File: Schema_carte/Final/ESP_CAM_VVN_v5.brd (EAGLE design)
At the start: 55.2 x 60.8 mm, 66 parts, among them M1 ELECTRET_MICROPHON-WM-62PC/62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, Q1 SI2305CDS, Q2 BSS131, Q3 SI2305CDS, Q6 SI2305CDS, Q7 BSS131, Q8 BSS131, U1 MCP3428-E/SL, U2 ESP32-WROVER-E, U3 PCA9685PW, U4 MIC5239-ADJMM, U5 MIC5239S, U6 MIC5239-ADJMM, X1 B2B-PH-K-S, X2 FH12-24S-0.5SH

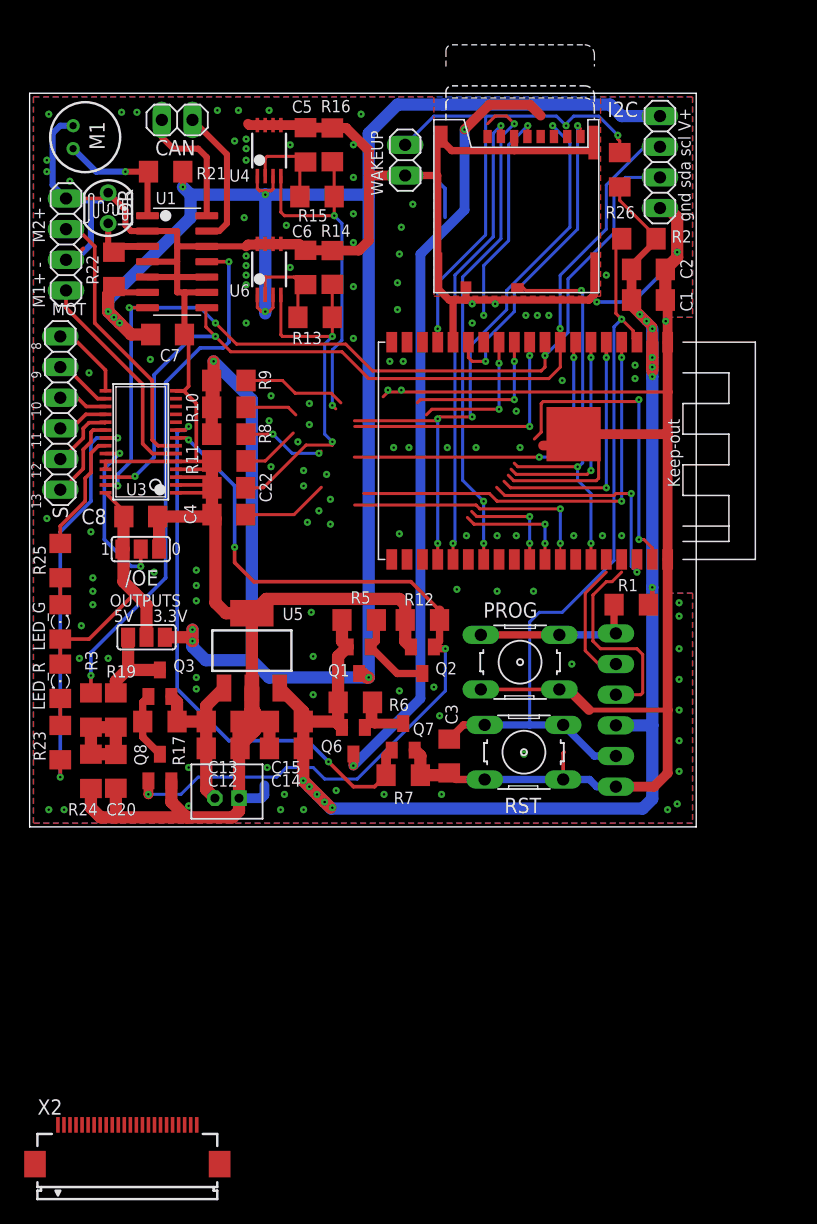
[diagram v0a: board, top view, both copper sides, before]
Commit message: romain maj
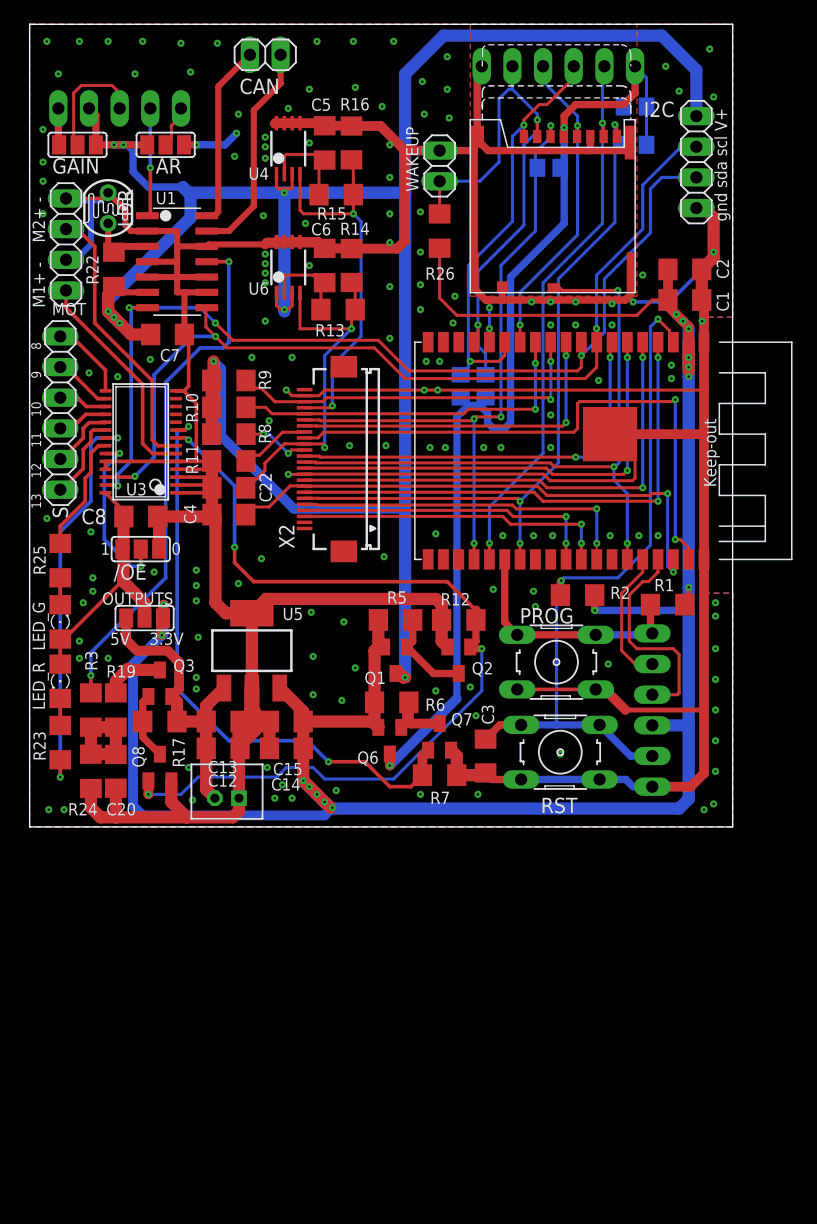
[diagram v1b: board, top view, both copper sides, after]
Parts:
- removed M1: ELECTRET_MICROPHON-WM-62PC/62PK, microphon:WM-62PC/62PK
- added AR, GAIN: (no value), jumper:SJ_2
- added MAX9814: (no value), pinhead:1X05
- added R18, R20, R27, R4: 47k, rcl:R0805
- added SD_SPI: (no value), pinhead:1X06
- R21: value 10k -> 47k; device eagle-ltspice:R1206 -> rcl:R0805
- moved X2 61.1 mm to (26.0, 30.5), turned to 90 degrees
- moved R21 39.3 mm to (50.2, 59.7), flipped to the bottom
- moved R2 30.0 mm to (45.4, 19.2)
- moved R26 15.8 mm to (34.0, 49.4)
- moved CAN 9.08 mm to (19.5, 64.0)
- moved R1 3.02 mm to (52.9, 18.4)
- moved C1 3.02 mm to (54.3, 43.7)
- moved C2 3.02 mm to (54.3, 46.2)
- moved C3 3.02 mm to (37.8, 5.87)
- moved I2C 3.02 mm to (55.2, 55.1)
- moved JP6 3.02 mm to (55.4, 9.68)
- moved PROG 3.02 mm to (43.7, 13.7)
- moved Q1 3.02 mm to (30.3, 13.8)
- moved Q2 3.02 mm to (35.6, 13.8)
- moved Q6 3.02 mm to (29.8, 7.14)
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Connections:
- removed net N$11: M1.2, R21.1, U1.1
- removed net SD_CLK: SD1.P$4
- new net AR: AR.2, MAX9814.1
- new net GAIN: GAIN.2, MAX9814.3
- new net N$2: MAX9814.2, U1.1
- net +5V: now also OUTPUTS.1
- net +5V/1: no longer OUTPUTS.1
- net CA_D0_SD_D1: now also R20.2
- net CA_PWDN_SD_CLK: now also SD1.P$4, SD_SPI.4
- net CA_RST_SD_CMD: now also R27.2
- net GND: now also AR.3, GAIN.1, MAX9814.5, SD_SPI.6; no longer M1.1
- net IO0: now also U2.IO0
- net RX: now also U2.RXD0; no longer U2.TXD0
- net SD_D0: now also R21.2, SD_SPI.2
- net SD_D2: now also R18.2, SD_SPI.3
- net SD_D3: now also R4.2, SD_SPI.5
- net TX: now also U2.TXD0; no longer U2.RXD0
- net V+: now also AR.1, GAIN.3, MAX9814.4; no longer OUTPUTS.3, R21.2
- net V+_SD: now also R18.1, R20.1, R21.1, R27.1, R4.1, SD_SPI.1
- net VCC: now also OUTPUTS.3
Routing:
- net VCC: track 118.2 -> 186.3 mm, vias 12 -> 15
- net GND: track 423.0 -> 452.0 mm, vias 124 -> 152
- net CA_PWDN_SD_CLK: track 0.00 -> 26.9 mm, vias 0 -> 2
- net CA_HREF: track 25.3 -> 47.2 mm
- net CA_XCLK_SD_DET: track 33.8 -> 54.2 mm
- net CA_D6: track 17.6 -> 37.7 mm
- net CA_D5: track 20.8 -> 40.3 mm
- net CA_D0_SD_D1: track 41.6 -> 59.4 mm
- net CA_PCLK: track 26.5 -> 44.1 mm
- net CA_D1: track 8.54 -> 25.4 mm
- net CA_D2: track 9.58 -> 26.1 mm
- net CA_SIO_C: track 16.2 -> 29.9 mm
- net N$11: track 10.7 -> 0.00 mm, vias 1 -> 0
- net +5V: track 14.7 -> 24.8 mm
- net GAIN: track 0.00 -> 10.0 mm
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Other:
- board size 55.2 x 60.8 mm -> 58.2 x 66.5 mm
- board text added: "AR OUT GAIN VCC GND"
- board text added: "ESP32_CAM_VVN V5.0"
- board text added: "M1 M2"
- board text added: "V+ cs mosi clk miso gnd"
- board text removed: "ESP32_CAM_VVN V4.0"
